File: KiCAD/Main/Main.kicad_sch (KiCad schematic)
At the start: 6 parts, among them J3 Conn_01x02_Socket, J6 Conn_01x02_Socket, J7 Conn_01x02_Socket, J8 Conn_01x02_Socket, U5 LT3092xST, U6 ADG5234BRUZ

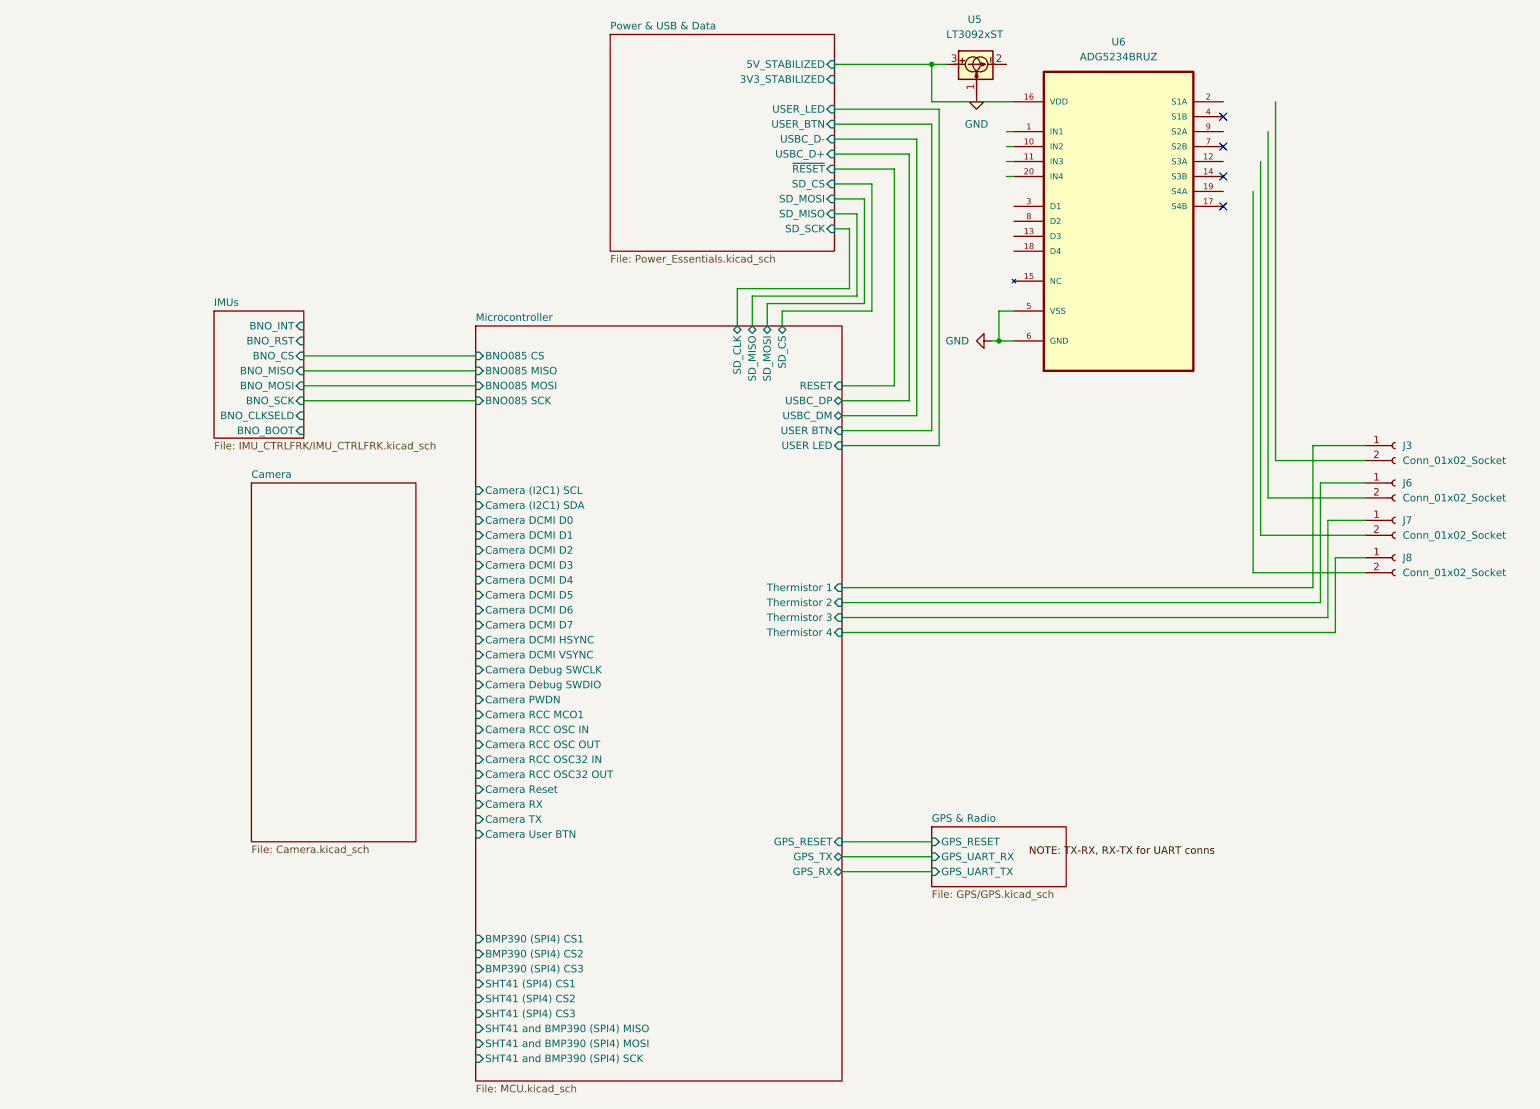
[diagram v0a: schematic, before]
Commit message: Add files via upload
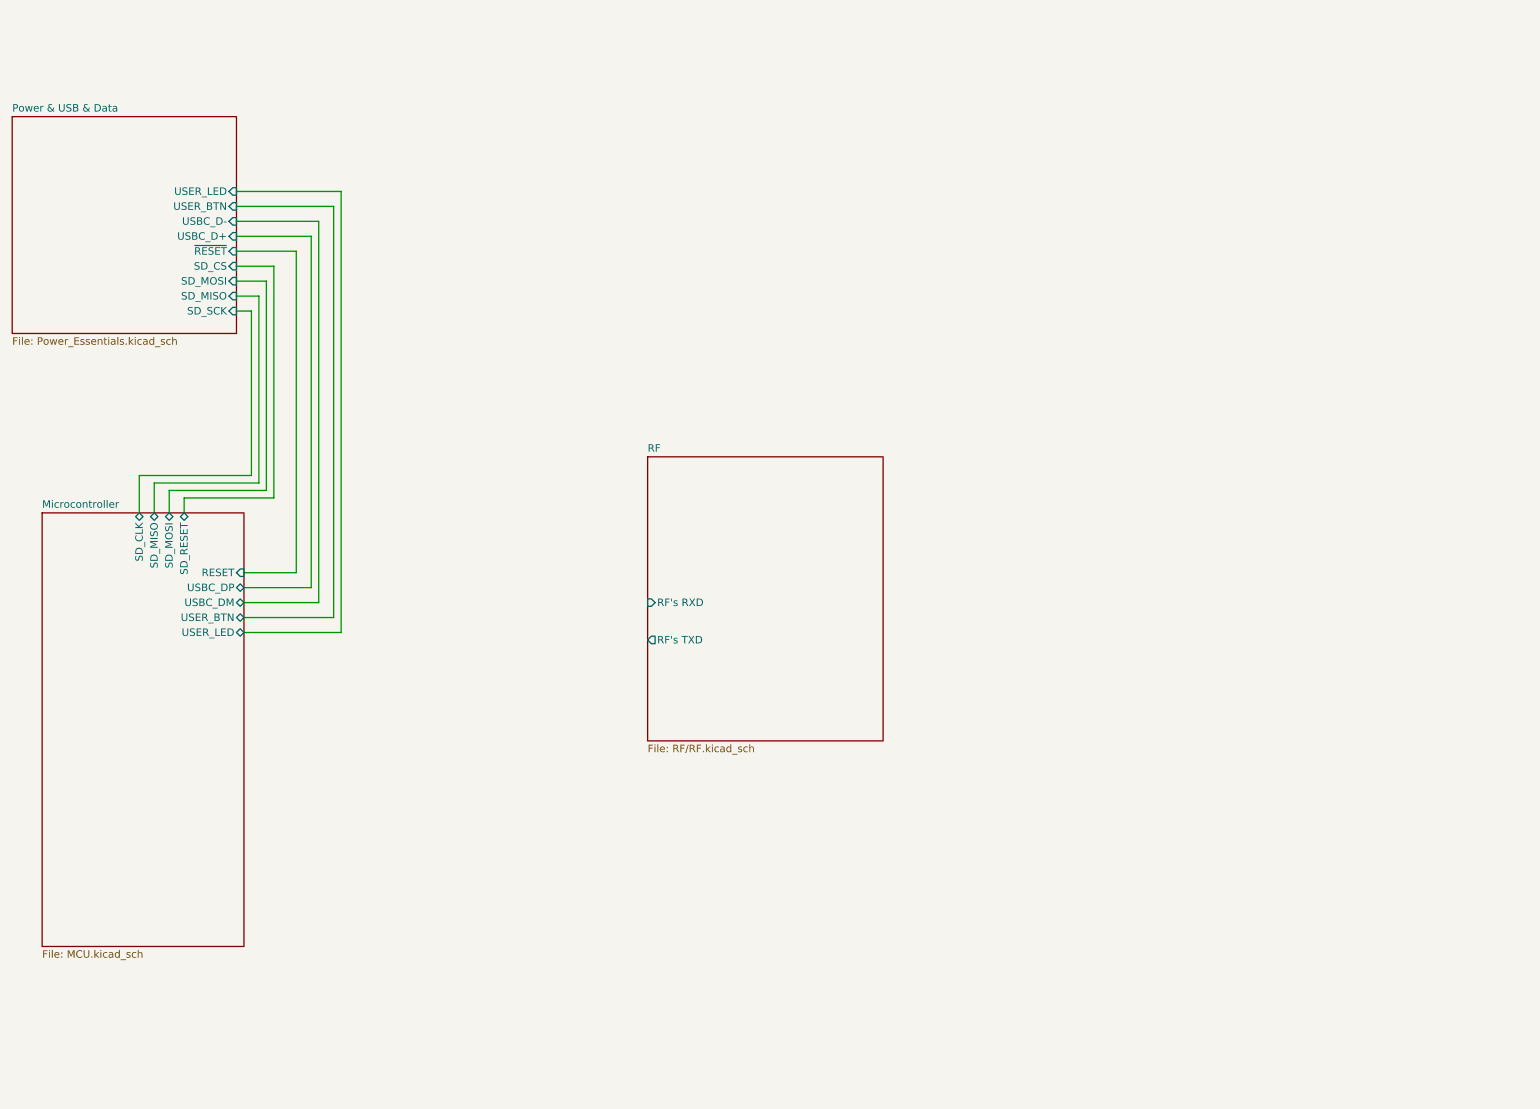
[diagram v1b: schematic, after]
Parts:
- removed J3, J6, J7, J8: Conn_01x02_Socket, symbol Connector:Conn_01x02_Socket
- removed U5: LT3092xST, Package_TO_SOT_SMD:SOT-223-3_TabPin2, symbol Reference_Current:LT3092xST
- removed U6: ADG5234BRUZ, ADG5234BRUZ:SOP65P640X120-20N, symbol ADG5234BRUZ:ADG5234BRUZ
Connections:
- no-connect marks 4 -> 0
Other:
- removed sheet Camera
- removed sheet GPS & Radio
- removed sheet IMUs
- added sheet RF (RF/RF.kicad_sch)
- sheet Microcontroller ports: added SD_RESET, USER_BTN, USER_LED; removed BMP390 (SPI4) CS1, BMP390 (SPI4) CS2, BMP390 (SPI4) CS3, BNO085 CS, BNO085 MISO, BNO085 MOSI, BNO085 SCK, Camera (I2C1) SCL, Camera (I2C1) SDA, Camera DCMI D0, Camera DCMI D1, Camera DCMI D2, Camera DCMI D3, Camera DCMI D4, Camera DCMI D5, Camera DCMI D6, Camera DCMI D7, Camera DCMI HSYNC, Camera DCMI VSYNC, Camera Debug SWCLK, Camera Debug SWDIO, Camera PWDN, Camera RCC MCO1, Camera RCC OSC IN, Camera RCC OSC OUT, Camera RCC OSC32 IN, Camera RCC OSC32 OUT, Camera RX, Camera Reset, Camera TX, Camera User BTN, GPS_RESET, GPS_RX, GPS_TX, SD_CS, SHT41 (SPI4) CS1, SHT41 (SPI4) CS2, SHT41 (SPI4) CS3, SHT41 and BMP390 (SPI4) MISO, SHT41 and BMP390 (SPI4) MOSI, SHT41 and BMP390 (SPI4) SCK, Thermistor 1, Thermistor 2, Thermistor 3, Thermistor 4, USER BTN, USER LED
- sheet Power & USB & Data ports: added none; removed 3V3_STABILIZED, 5V_STABILIZED
